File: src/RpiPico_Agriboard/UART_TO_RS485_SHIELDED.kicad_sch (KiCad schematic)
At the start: 11 parts, among them J19 Screw_Terminal_01x03, U10 TBU-CA065-200-WH, U11 TBU-CA065-200-WH, U8 TP8485E-SR

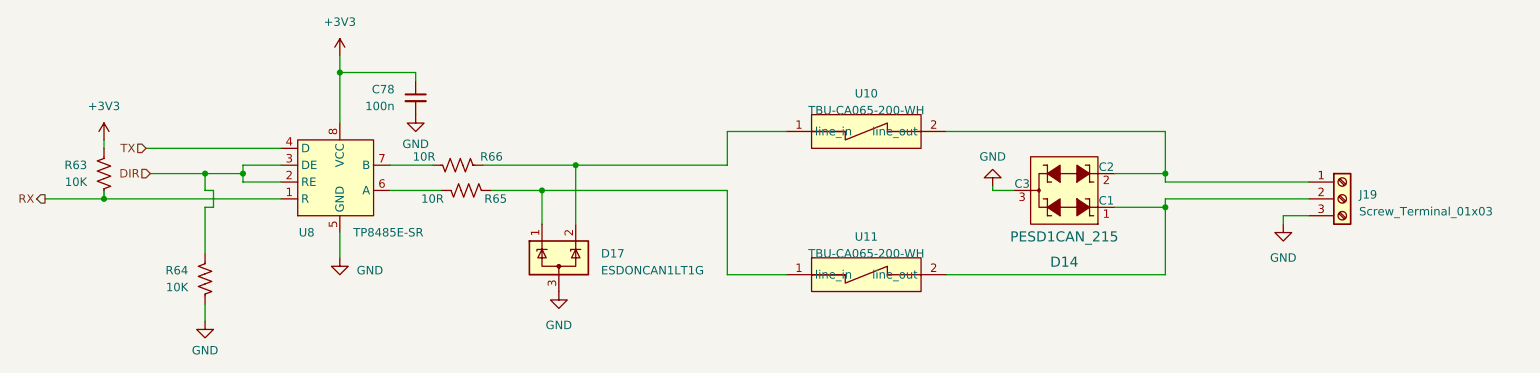
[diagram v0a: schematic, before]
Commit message: rs485 updates and layout updates
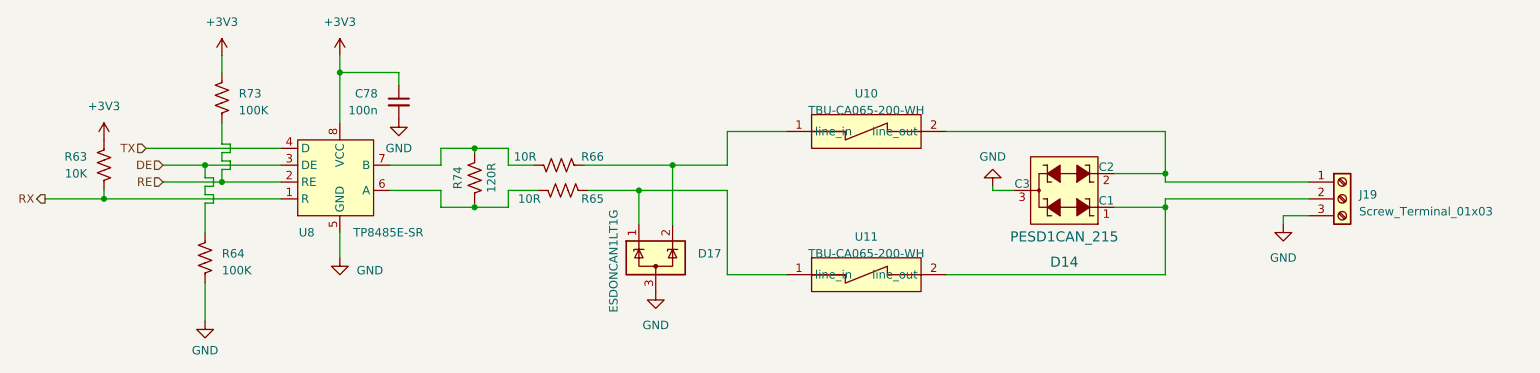
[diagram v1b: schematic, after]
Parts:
- added R73: 100K, Resistor_SMD:R_0402_1005Metric, symbol Device:R_US
- added R74: 120R, Resistor_SMD:R_0402_1005Metric, symbol Device:R_US
- R64: value 10K -> 100K
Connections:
- net +3V3: now also R73.1
- net at R65.1, U8.6 (A): now also R74.1
- net at R66.1, U8.7 (B): now also R74.2
- net DIR renamed DE
- net DE: no longer U8.2 (RE)
- new net RE: R73.2, U8.2 (RE)
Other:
- moved on the sheet: C78, D17, R63, R64, R65, R66
